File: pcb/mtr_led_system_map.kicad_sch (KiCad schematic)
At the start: 431 parts, among them J1 USB_C_Receptacle_USB2.0_16P, U1 ESP32-S3-WROOM-1, U2 AP2112K-3.3

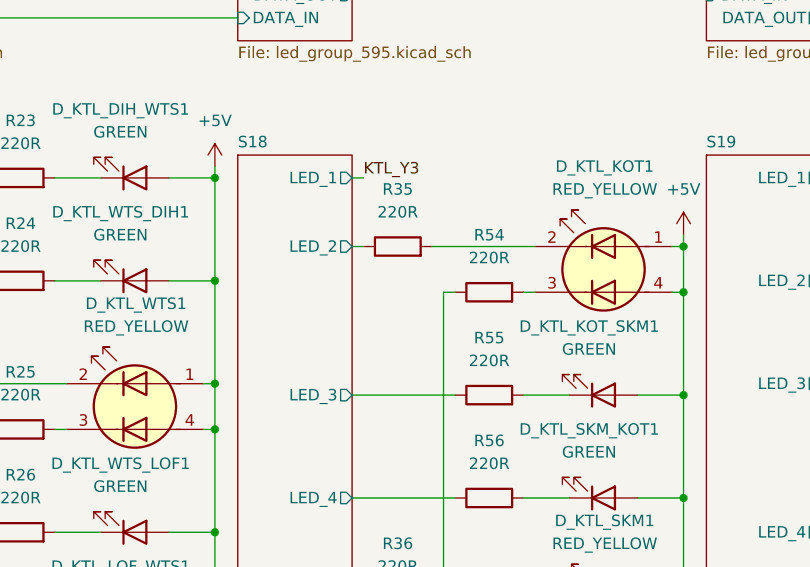
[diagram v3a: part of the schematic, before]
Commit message: PCB track routing part 4
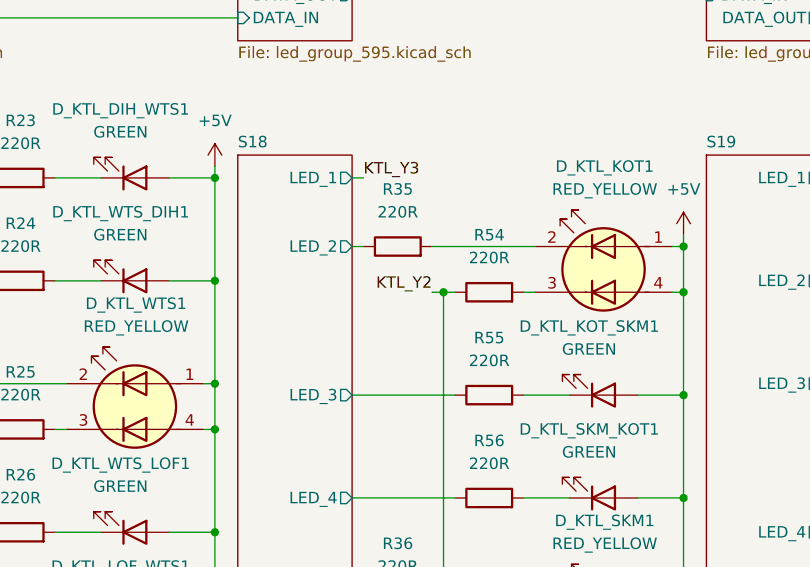
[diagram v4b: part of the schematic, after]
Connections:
- net KTL_Y2: now also R54.1, R57.1, R60.1
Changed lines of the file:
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@@
 	)
 	(junction
+		(at 100.33 269.24)
+		(diameter 0)
+		(color 0 0 0 0)
+	)
+	(junction
 		(at 127 303.53)
 		(diameter 0)
@@
 	(wire
 		(pts
+			(xy 99.06 269.24) (xy 100.33 269.24)
+		)
+		(stroke
+			(width 0)
+			(type default)
+		)
+	)
+	(wire
+		(pts
 			(xy 142.24 346.71) (xy 153.67 346.71)
 		)
@@
 		)
 	)
+	(label "KTL_Y2"
+		(at 99.06 269.24 180)
+		(effects
+			(font
+				(size 1.27 1.27)
+			)
+			(justify right bottom)
+		)
+	)

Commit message: PCB track routing part 5
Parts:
- removed R241, R242: 33R, Resistor_SMD:R_0603_1608Metric, symbol Device:R
- renumbered R188 to R100, R189 to R101, R190 to R102, R191 to R103, R192 to R104, R193 to R105, R108 to R106, R109 to R107, R110 to R108, R111 to R109, R112 to R110, R113 to R111, R114 to R112, R115 to R113, R16 to R114, R17 to R115, R18 to R116, R19 to R117, R20 to R118, R21 to R119, R22 to R120, R61 to R121, R62 to R122, R63 to R123, R64 to R124, R65 to R125, R66 to R126, R67 to R127, R70 to R128, R71 to R129, R72 to R130, R73 to R131, R74 to R132, R75 to R133, R76 to R134, R77 to R135, R78 to R136, R79 to R137, R80 to R138, R81 to R139, R82 to R140, R83 to R141, R84 to R142, R229 to R143, R230 to R144, R231 to R145, R232 to R146, R233 to R147, R234 to R148, R235 to R149, R236 to R150, R210 to R153, R211 to R154, R212 to R155, R158 to R156, R159 to R157, R160 to R158, R161 to R159, R54 to R16, R162 to R160, R163 to R161, R164 to R162, R165 to R163, R220 to R164, R221 to R165, R222 to R166, R223 to R167, R224 to R168, R225 to R169, R55 to R17, R226 to R170, R93 to R171, R94 to R172, R205 to R173, R206 to R174, R100 to R175, R101 to R176, R102 to R177, R103 to R178, R104 to R179, R56 to R18, R105 to R180, R106 to R181, R107 to R182, R227 to R183, R228 to R184, R123 to R185, R124 to R186, R125 to R187, R186 to R188, R131 to R189, R57 to R19, R132 to R190, R133 to R191, R134 to R192, R135 to R193, R136 to R194, R137 to R195, R202 to R196, R203 to R197, R204 to R198, R237 to R199, R58 to R20, R238 to R200, R126 to R201, R127 to R202, R184 to R203, R185 to R204, R138 to R205, R139 to R206, R140 to R207, R141 to R208, R142 to R209, R59 to R21, R143 to R210, R194 to R211, R195 to R212, R196 to R213, R197 to R214, R198 to R215, R199 to R216, R200 to R217, R201 to R218, R239 to R219, R60 to R22, R240 to R220, R243 to R221, R244 to R222, R245 to R223, R68 to R224, R69 to R225, R153 to R226, R154 to R227, R155 to R228, R246 to R229, R46 to R23, R85 to R230, R86 to R231, R87 to R232, R88 to R233, R89 to R234, R90 to R235, R91 to R236, R92 to R237, R166 to R238, R167 to R239, R47 to R24, R168 to R240, R169 to R241, R170 to R242, R171 to R243, R172 to R244, R48 to R25, R49 to R26, R50 to R27, R51 to R28, R52 to R29, R53 to R30, R7 to R33, R8 to R34, R156 to R35, R157 to R36, R38 to R37, R39 to R38, R40 to R39, R35 to R4, R41 to R40, R42 to R41, R43 to R42, R44 to R43, R45 to R44, R23 to R45, R24 to R46, R25 to R47, R26 to R48, R27 to R49, R36 to R5, R28 to R50, R29 to R51, R30 to R52, R173 to R53, R174 to R54, R175 to R55, R176 to R56, R177 to R57, R178 to R58, R179 to R59, R37 to R6, R180 to R60, R207 to R61, R208 to R62, R209 to R63, R97 to R64, R98 to R65, R99 to R66, R128 to R67, R129 to R68, R130 to R69, R33 to R7, R213 to R70, R214 to R71, R215 to R72, R216 to R73, R217 to R74, R218 to R75, R219 to R76, R116 to R77, R117 to R78, R118 to R79, R34 to R8, R119 to R80, R120 to R81, R121 to R82, R122 to R83, R144 to R84, R145 to R85, R146 to R86, R147 to R87, R148 to R88, R149 to R89, R150 to R90, R181 to R91, R182 to R92, R183 to R93, R95 to R94, R96 to R95, R4 to R96, R5 to R97, R6 to R98, R187 to R99
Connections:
- net +5V: no longer D_DOOR_G1.2 (A), D_DOOR_Y1.2 (A)
- new net: D_DOOR_G1.2 (A), D_DOOR_Y1.2 (A)
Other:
- sheet S16 ports: added DATA_OUT; removed none
- sheet S24 ports: added DATA_OUT; removed none
- sheet S8 ports: added DATA_OUT; removed none
- sheet S9 ports: added none; removed DATA_OUT
- moved on the sheet: C1, C2, C3, C4, C5, C6, D_DOOR_G1, D_DOOR_Y1, D_ISL_CEN1, D_ISL_CEN_SHW1, D_ISL_CHW1, D_ISL_CHW_HFC1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
